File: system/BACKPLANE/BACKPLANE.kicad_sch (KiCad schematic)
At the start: 81 parts, among them J1 BusConnector, J10 BusConnector, J11 BusConnector, J12 BusConnector, J13 BusConnector, J14 BusConnector, J15 BusConnector, J16 BusConnector, J17 BusConnector, J18 BusConnector, J19 BusConnector, J2 BusConnector, J20 BusConnector, J29 ATX-24, J3 BusConnector, J30 ATX-04, J4 BusConnector, J5 BusConnector, J6 BusConnector, J7 BusConnector, J8 BusConnector, J9 BusConnector

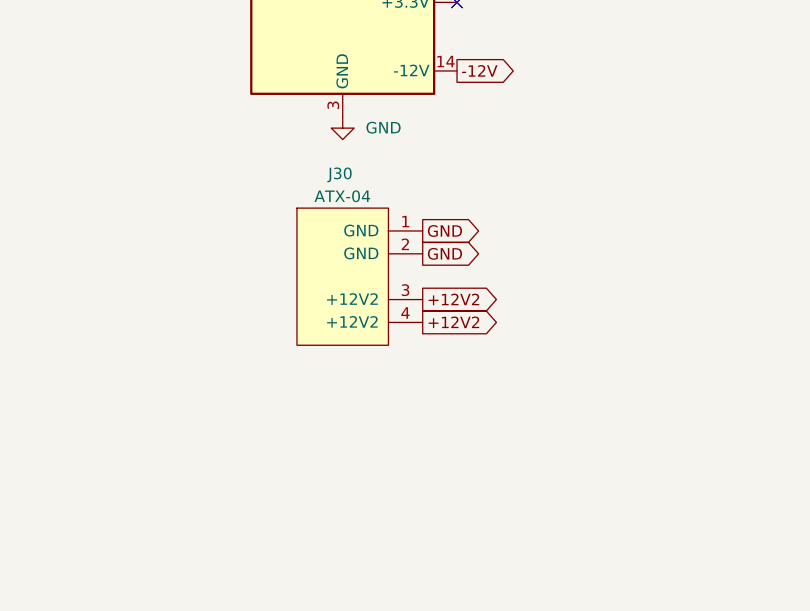
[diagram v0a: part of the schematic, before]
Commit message: backplane pcb
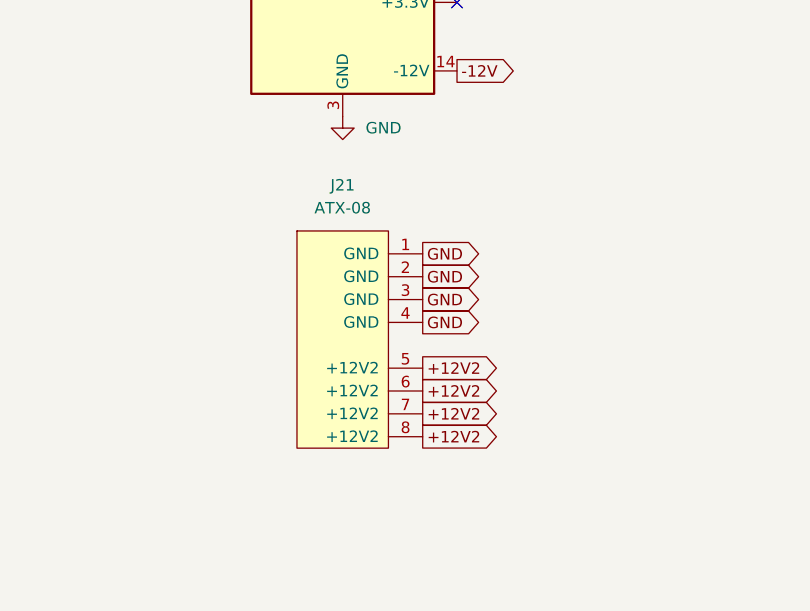
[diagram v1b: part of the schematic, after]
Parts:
- removed J30: ATX-04, IMNOTWOPR:ATX-04, symbol IMNOTWOPR:ATX-04
- added J21: ATX-08, IMNOTWOPR:ATX-08, symbol IMNOTWOPR:ATX-08
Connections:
- net +12V2: now also J21.5 (+12V2), J21.6 (+12V2), J21.7 (+12V2), J21.8 (+12V2)
- net GND: now also J21.1 (GND), J21.2 (GND), J21.3 (GND), J21.4 (GND)
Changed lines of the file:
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@@
 	(global_label "+12V2"
 		(shape output)
-		(at 513.08 359.41 0)
+		(at 513.08 367.03 0)
 		(fields_autoplaced yes)
 		(effects
@@
 		)
 		(property "Intersheetrefs" "${INTERSHEET_REFS}"
-			(at 522.3547 359.41 0)
+			(at 522.3547 367.03 0)
 			(hide yes)
 			(show_name no)
@@
 		)
 	)
+	(global_label "+12V2"
+		(shape output)
+		(at 513.08 374.65 0)
+		(fields_autoplaced yes)
+		(effects
+			(font
+				(size 1.27 1.27)
+			)
+			(justify left)
+		)
+		(property "Intersheetrefs" "${INTERSHEET_REFS}"
+			(at 522.3547 374.65 0)
+			(hide yes)
+			(show_name no)
+			(do_not_autoplace no)
+			(effects
+				(font
+					(size 1.27 1.27)
+				)
+				(justify left)
+			)
+		)
+	)
 	(global_label "b27"
 		(shape passive)
@@
 		)
 	)
+	(global_label "GND"
+		(shape output)
+		(at 513.08 359.41 0)
+		(fields_autoplaced yes)
+		(effects
+			(font
+				(size 1.27 1.27)
+			)
+			(justify left)
+		)
+		(property "Intersheetrefs" "${INTERSHEET_REFS}"
+			(at 519.9357 359.41 0)
+			(hide yes)
+			(show_name no)
+			(do_not_autoplace no)
+			(effects
+				(font
+					(size 1.27 1.27)
+				)
+				(justify left)
+			)
+		)
+	)
 	(global_label "+5VSB"
 		(shape input)
@@
 	(global_label "GND"
 		(shape output)
-		(at 513.08 354.33 0)
+		(at 513.08 356.87 0)
 		(fields_autoplaced yes)
 		(effects
@@
 		)
 		(property "Intersheetrefs" "${INTERSHEET_REFS}"
-			(at 519.9357 354.33 0)
+			(at 519.9357 356.87 0)
 			(hide yes)
 			(show_name no)
@@
 	)
 	(global_label "GND"
+		(shape output)
+		(at 513.08 361.95 0)
+		(fields_autoplaced yes)
+		(effects
+			(font
+				(size 1.27 1.27)
+			)
+			(justify left)
+		)
+		(property "Intersheetrefs" "${INTERSHEET_REFS}"
+			(at 519.9357 361.95 0)
+			(hide yes)
+			(show_name no)
+			(do_not_autoplace no)
+			(effects
+				(font
+					(size 1.27 1.27)
+				)
+				(justify left)
+			)
+		)
+	)
+	(global_label "GND"
 		(shape passive)
 		(at 703.58 116.84 180)
@@
 		)
 	)
+	(global_label "+12V2"
+		(shape output)
+		(at 513.08 372.11 0)
+		(fields_autoplaced yes)
+		(effects
+			(font
+				(size 1.27 1.27)
+			)
+			(justify left)
+		)
+		(property "Intersheetrefs" "${INTERSHEET_REFS}"
+			(at 522.3547 372.11 0)
+			(hide yes)
+			(show_name no)
+			(do_not_autoplace no)
+			(effects
+				(font
+					(size 1.27 1.27)
+				)
+				(justify left)
+			)
+		)
+	)
 	(global_label "GND"
 		(shape passive)
@@
 	(global_label "GND"
 		(shape output)
-		(at 513.08 351.79 0)
+		(at 513.08 354.33 0)
 		(fields_autoplaced yes)
 		(effects
@@
 		)
 		(property "Intersheetrefs" "${INTERSHEET_REFS}"
-			(at 519.9357 351.79 0)
+			(at 519.9357 354.33 0)
 			(hide yes)
 			(show_name no)
@@
 	(global_label "+12V2"
 		(shape output)
-		(at 513.08 361.95 0)
+		(at 513.08 369.57 0)
 		(fields_autoplaced yes)
 		(effects
@@
 		)
 		(property "Intersheetrefs" "${INTERSHEET_REFS}"
-			(at 522.3547 361.95 0)
+			(at 522.3547 369.57 0)
 			(hide yes)
 			(show_name no)
@@
 	)
 	(symbol
+		(lib_id "IMNOTWOPR:ATX-08")
+		(at 504.19 358.14 0)
+		(unit 1)
+		(body_style 1)
+		(exclude_from_sim no)
+		(in_bom yes)
+		(on_board yes)
+		(in_pos_files yes)
+		(dnp no)
+		(fields_autoplaced yes)
+		(property "Reference" "J21"
+			(at 504.19 346.71 0)
+			(show_name no)
+			(do_not_autoplace no)
+			(effects
+				(font
+					(size 1.27 1.27)
+				)
+			)
+		)
+		(property "Value" "ATX-08"
+			(at 504.19 349.25 0)
+			(show_name no)
+			(do_not_autoplace no)
+			(effects
+				(font
+					(size 1.27 1.27)
+				)
+			)
+		)
+		(property "Footprint" "IMNOTWOPR:ATX-08"
+			(at 504.19 358.14 0)
+			(hide yes)
+			(show_name no)
+			(do_not_autoplace no)
+			(effects
+				(font
+					(size 1.27 1.27)
+				)
+			)
+		)
+		(property "Datasheet" ""
+			(at 504.19 358.14 0)
+			(hide yes)
+			(show_name no)
+			(do_not_autoplace no)
+			(effects
+				(font
+					(size 1.27 1.27)
+				)
+			)
+		)
+		(property "Description" "Generic connector, double row, 02x02, top/bottom pin numbering scheme (row 1: 1...pins_per_row, row2: pins_per_row+1 ... num_pins), script generated (kicad-library-utils/schlib/autogen/connector/)"
+			(at 504.19 358.14 0)
+			(hide yes)
+			(show_name no)
+			(do_not_autoplace no)
+			(effects
+				(font
+					(size 1.27 1.27)
+				)
+			)
+		)
+		(pin "6"
+		)
+		(pin "5"
+		)
+		(pin "4"
+		)
+		(pin "1"
+		)
+		(pin "2"
+		)
+		(pin "7"
+		)
+		(pin "3"
+		)
+		(pin "8"
+		)
+		(instances
+			(project "BACKPLANE"
+				(path "/ad2d789c-a8c8-48c5-8f34-468c01c0c6c9"
+					(reference "J21")
+					(unit 1)
+				)
+			)
+		)
+	)
+	(symbol
 		(lib_id "IMNOTWOPR:BusConnector")
 		(at 124.46 241.3 0)
@@
 					(unit 1)
 				)
-			)
-		)
-	)
-	(symbol
-		(lib_id "IMNOTWOPR:ATX-04")
-		(at 504.19 355.6 0)
-		(unit 1)
-		(body_style 1)
-		(exclude_from_sim no)
-		(in_bom yes)
-		(on_board yes)
-		(in_pos_files yes)
-		(dnp no)
-		(property "Reference" "J30"
-			(at 503.936 345.44 0)
-			(show_name no)
-			(do_not_autoplace no)
-			(effects
-				(font
-					(size 1.27 1.27)
-				)
-			)
-		)
-		(property "Value" "ATX-04"
-			(at 504.19 347.98 0)
-			(show_name no)
-			(do_not_autoplace no)
-			(effects
-				(font
-					(size 1.27 1.27)
-				)
-			)
-		)
-		(property "Footprint" "IMNOTWOPR:ATX-04"
-			(at 504.19 355.6 0)
-			(hide yes)
-			(show_name no)
-			(do_not_autoplace no)
-			(effects
-				(font
-					(size 1.27 1.27)
-				)
-			)
-		)
-		(property "Datasheet" ""
-			(at 504.19 355.6 0)
-			(hide yes)
-			(show_name no)
-			(do_not_autoplace no)
-			(effects
-				(font
-					(size 1.27 1.27)
-				)
-			)
-		)
-		(property "Description" "Generic connector, double row, 02x02, top/bottom pin numbering scheme (row 1: 1...pins_per_row, row2: pins_per_row+1 ... num_pins), script generated (kicad-library-utils/schlib/autogen/connector/)"
-			(at 504.19 355.6 0)
-			(hide yes)
-			(show_name no)
-			(do_not_autoplace no)
-			(effects
-				(font
-					(size 1.27 1.27)
-				)
-			)
-		)
-		(pin "4"
-		)
-		(pin "3"
-		)
-		(pin "2"
-		)
-		(pin "1"
-		)
-		(instances
-			(project "BACKPLANE"
-				(path "/ad2d789c-a8c8-48c5-8f34-468c01c0c6c9"
-					(reference "J30")
-					(unit 1)
-				)
